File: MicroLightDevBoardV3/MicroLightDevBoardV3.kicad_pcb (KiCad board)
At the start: 6 copper layers, 12.5 x 18 mm, 34 parts, among them J1 TYPE-C-31-M-12, J3 Conn_01x03_Socket, J4 Conn_01x01_Socket, J5 Conn_01x01_Socket, J6 Conn_01x04_Socket, SW1 SW_Push, U1 USBLC6-2P6, U2 STM32C071GBUx, U3 BQ25180, U4 S-85S1AB33-I6T1U, U5 DF53-2S-0.6H, U7 MC3479

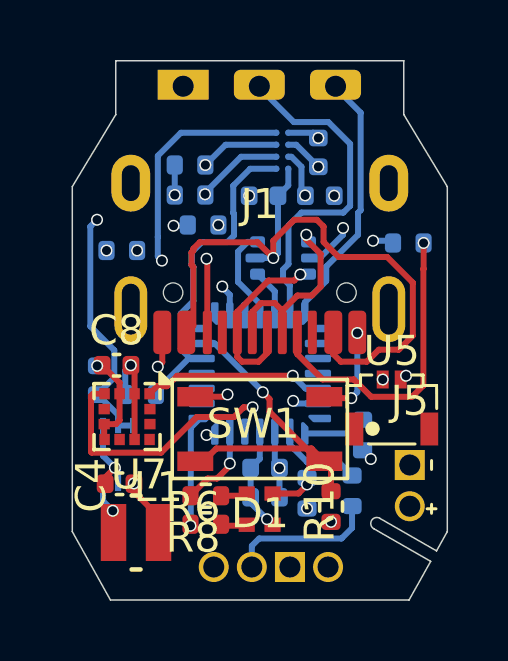
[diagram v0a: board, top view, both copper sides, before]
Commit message: cleanup traces
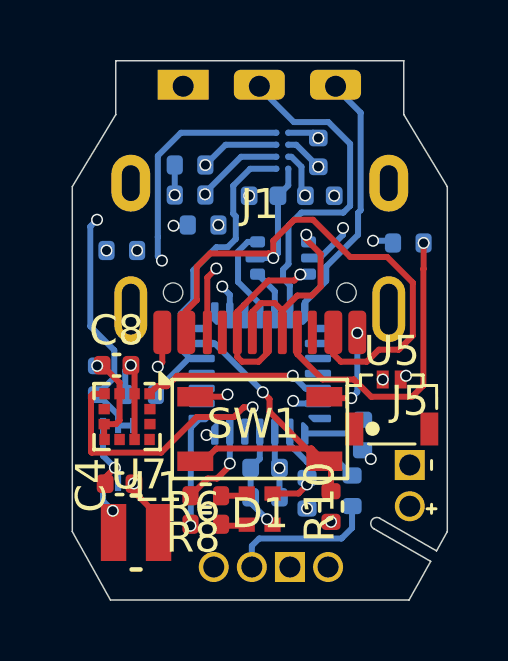
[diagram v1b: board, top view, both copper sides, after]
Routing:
- net VBUS_CHRG: track 22.0 -> 20.9 mm
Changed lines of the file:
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@@
 	)
 	(segment
-		(start 47.474 23.917479)
-		(end 47.536 23.855479)
+		(start 47.649 24.392479)
+		(end 48.092479 23.949)
+		(width 0.2)
+		(layer "F.Cu")
+		(net 1)
+	)
+	(segment
+		(start 54.851 26.686785)
+		(end 54.851 24.923215)
+		(width 0.2)
+		(layer "F.Cu")
+		(net 1)
+	)
+	(segment
+		(start 48.092479 23.949)
+		(end 50.049 23.949)
+		(width 0.2)
+		(layer "F.Cu")
+		(net 1)
+	)
+	(segment
+		(start 47.3 25.855001)
+		(end 47.649 25.506001)
+		(width 0.2)
+		(layer "F.Cu")
+		(net 1)
+	)
+	(segment
+		(start 47.3 26.58)
+		(end 47.3 25.855001)
 		(width 0.2)
 		(layer "F.Cu")
@@
 	)
 	(segment
-		(start 47.536 26.344)
-		(end 47.536 24.394521)
-		(width 0.2)
-		(layer "F.Cu")
-		(net 1)
-	)
-	(segment
-		(start 51.876 23.567112)
-		(end 51.876 23.051)
-		(width 0.2)
-		(layer "F.Cu")
-		(net 1)
-	)
-	(segment
-		(start 51.876 23.051)
-		(end 51.65 22.825)
-		(width 0.2)
-		(layer "F.Cu")
-		(net 1)
-	)
-	(segment
-		(start 47.536 23.855479)
-		(end 47.536 23.789)
-		(width 0.2)
-		(layer "F.Cu")
-		(net 1)
-	)
-	(segment
-		(start 47.536 24.394521)
-		(end 47.474 24.332521)
-		(width 0.2)
-		(layer "F.Cu")
-		(net 1)
-	)
-	(segment
-		(start 47.75 23.575)
-		(end 49.675 23.575)
-		(width 0.2)
-		(layer "F.Cu")
-		(net 1)
-	)
-	(segment
-		(start 52.376 24.067112)
-		(end 51.876 23.567112)
+		(start 50.9 22.825)
+		(end 50.2 23.525)
+		(width 0.2)
+		(layer "F.Cu")
+		(net 1)
+	)
+	(segment
+		(start 53.318215 27.556)
+		(end 53.718215 27.156)
+		(width 0.2)
+		(layer "F.Cu")
+		(net 1)
+	)
+	(segment
+		(start 47.649 25.506001)
+		(end 47.649 24.392479)
+		(width 0.2)
+		(layer "F.Cu")
+		(net 1)
+	)
+	(segment
+		(start 54.381785 27.156)
+		(end 54.851 26.686785)
+		(width 0.2)
+		(layer "F.Cu")
+		(net 1)
+	)
+	(segment
+		(start 50.049 23.949)
+		(end 50.2 24.1)
+		(width 0.2)
+		(layer "F.Cu")
+		(net 1)
+	)
+	(segment
+		(start 52.2 26.58)
+		(end 52.2 27.304999)
+		(width 0.2)
+		(layer "F.Cu")
+		(net 1)
+	)
+	(segment
+		(start 52.451001 27.556)
+		(end 53.318215 27.556)
+		(width 0.2)
+		(layer "F.Cu")
+		(net 1)
+	)
+	(segment
+		(start 52.2 27.304999)
+		(end 52.451001 27.556)
+		(width 0.2)
+		(layer "F.Cu")
+		(net 1)
+	)
+	(segment
+		(start 53.994897 24.067112)
+		(end 52.767112 24.067112)
 		(width 0.2)
 		(layer "F.Cu")
@@
 	)
 	(segment
-		(start 52.451001 27.556)
-		(end 52.2 27.304999)
-		(width 0.2)
-		(layer "F.Cu")
-		(net 1)
-	)
-	(segment
-		(start 47.474 24.332521)
-		(end 47.474 23.917479)
-		(width 0.2)
-		(layer "F.Cu")
-		(net 1)
-	)
-	(segment
-		(start 50.9 22.825)
-		(end 50.2 23.525)
-		(width 0.2)
-		(layer "F.Cu")
-		(net 1)
-	)
-	(segment
-		(start 53.318215 27.556)
-		(end 52.451001 27.556)
+		(start 51.525 22.825)
+		(end 50.9 22.825)
 		(width 0.2)
 		(layer "F.Cu")
@@
 	)
 	(segment
-		(start 47.3 26.58)
-		(end 47.536 26.344)
-		(width 0.2)
-		(layer "F.Cu")
-		(net 1)
-	)
-	(segment
-		(start 49.675 23.575)
-		(end 50.2 24.1)
-		(width 0.2)
-		(layer "F.Cu")
-		(net 1)
-	)
-	(segment
-		(start 54.851 26.686785)
-		(end 54.851 24.923215)
-		(width 0.2)
-		(layer "F.Cu")
-		(net 1)
-	)
-	(segment
-		(start 47.536 23.789)
-		(end 47.75 23.575)
-		(width 0.2)
-		(layer "F.Cu")
-		(net 1)
-	)
-	(segment
-		(start 54.381785 27.156)
-		(end 54.851 26.686785)
-		(width 0.2)
-		(layer "F.Cu")
-		(net 1)
-	)
-	(segment
-		(start 53.994897 24.067112)
-		(end 52.376 24.067112)
-		(width 0.2)
-		(layer "F.Cu")
-		(net 1)
-	)
-	(segment
-		(start 53.718215 27.156)
-		(end 53.318215 27.556)
-		(width 0.2)
-		(layer "F.Cu")
-		(net 1)
-	)
-	(segment
-		(start 52.2 27.304999)
-		(end 52.2 26.58)
-		(width 0.2)
-		(layer "F.Cu")
-		(net 1)
-	)
-	(segment
-		(start 51.65 22.825)
-		(end 50.9 22.825)
+		(start 52.767112 24.067112)
+		(end 51.525 22.825)
 		(width 0.2)
 		(layer "F.Cu")
@@
 	)
 	(segment
-		(start 48 24.15)
-		(end 47.975 24.125)
+		(start 48.3 24.45)
+		(end 48 24.75)
 		(width 0.2)
 		(layer "F.Cu")
@@
 	)
 	(segment
-		(start 48 26.58)
-		(end 48 24.15)
+		(start 48 24.75)
+		(end 48 26.58)
 		(width 0.2)
 		(layer "F.Cu")
@@
 	)
 	(via
-		(at 47.975 24.125)
+		(at 48.3 24.45)
 		(size 0.4)
 		(drill 0.3)
@@
 	(segment
 		(start 46.875 23.025)
-		(end 47.975 24.125)
+		(end 48.3 24.45)
 		(width 0.2)
 		(layer "In2.Cu")
@@
 	)
 	(segment
-		(start 48.864 22.602)
-		(end 48.864 21.689162)
+		(start 47.114 25.956008)
+		(end 47.536 25.534008)
+		(width 0.2)
+		(layer "B.Cu")
+		(net 27)
+	)
+	(segment
+		(start 48.864 22.624372)
+		(end 48.95 22.710372)
+		(width 0.2)
+		(layer "B.Cu")
+		(net 27)
+	)
+	(segment
+		(start 47.8125 27.45)
+		(end 47.429912 27.45)
 		(width 0.2)
 		(layer "B.Cu")
@@
 	)
 	(segment
-		(start 48.891 22.629)
-		(end 48.864 22.602)
+		(start 46.285 28.543612)
+		(end 47.378612 27.45)
+		(width 0.2)
+		(layer "B.Cu")
+		(net 27)
+	)
+	(segment
+		(start 48.864 21.689162)
+		(end 48.864 22.624372)
+		(width 0.2)
+		(layer "B.Cu")
+		(net 27)
+	)
+	(segment
+		(start 48.673 23.7425)
+		(end 48.298979 23.7425)
+		(width 0.2)
+		(layer "B.Cu")
+		(net 27)
+	)
+	(segment
+		(start 47.429912 27.45)
+		(end 47.114 27.134088)
 		(width 0.2)
 		(layer "B.Cu")
@@
 	)
 	(segment
+		(start 48.95 23.4655)
+		(end 48.673 23.7425)
+		(width 0.2)
+		(layer "B.Cu")
+		(net 27)
+	)
+	(segment
+		(start 48.864 21.689162)
+		(end 49.428162 21.125)
+		(width 0.2)
+		(layer "B.Cu")
+		(net 27)
+	)
+	(segment
+		(start 48.95 22.710372)
+		(end 48.95 23.4655)
+		(width 0.2)
+		(layer "B.Cu")
+		(net 27)
+	)
+	(segment
 		(start 49.428162 21.125)
 		(end 50.3 21.125)
@@
 	)
 	(segment
-		(start 47.474 23.917479)
-		(end 47.820479 23.571)
+		(start 47.536 24.505479)
+		(end 47.536 25.534008)
 		(width 0.2)
 		(layer "B.Cu")
@@
 	)
 	(segment
-		(start 47.474 24.332521)
-		(end 47.474 23.917479)
-		(width 0.2)
-		(layer "B.Cu")
-		(net 27)
-	)
-	(segment
-		(start 46.285 28.543612)
-		(end 47.378612 27.45)
-		(width 0.2)
-		(layer "B.Cu")
-		(net 27)
-	)
-	(segment
-		(start 48.891 23.348628)
-		(end 48.891 22.629)
-		(width 0.2)
-		(layer "B.Cu")
-		(net 27)
-	)
-	(segment
-		(start 48.668628 23.571)
-		(end 48.891 23.348628)
-		(width 0.2)
-		(layer "B.Cu")
-		(net 27)
-	)
-	(segment
-		(start 47.8125 27.45)
-		(end 47.429912 27.45)
-		(width 0.2)
-		(layer "B.Cu")
-		(net 27)
-	)
-	(segment
-		(start 48.864 21.689162)
-		(end 49.428162 21.125)
-		(width 0.2)
-		(layer "B.Cu")
-		(net 27)
-	)
-	(segment
-		(start 47.536 25.534008)
-		(end 47.536 24.394521)
-		(width 0.2)
-		(layer "B.Cu")
-		(net 27)
-	)
-	(segment
-		(start 47.536 24.394521)
-		(end 47.474 24.332521)
-		(width 0.2)
-		(layer "B.Cu")
-		(net 27)
-	)
-	(segment
-		(start 47.820479 23.571)
-		(end 48.668628 23.571)
-		(width 0.2)
-		(layer "B.Cu")
-		(net 27)
-	)
-	(segment
-		(start 47.429912 27.45)
-		(end 47.114 27.134088)
-		(width 0.2)
-		(layer "B.Cu")
-		(net 27)
-	)
-	(segment
-		(start 47.114 25.956008)
-		(end 47.536 25.534008)
-		(width 0.2)
-		(layer "B.Cu")
+		(start 48.298979 23.7425)
+		(end 47.536 24.505479)
+		(width 0.2)
+		(layer "B.Cu")
